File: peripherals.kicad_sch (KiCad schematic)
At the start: 20 parts, among them J2 Pad, Q1 MMBT3904, SW1 DSHP02TSGET, U2 BH1750FVI, U4 SHTC3

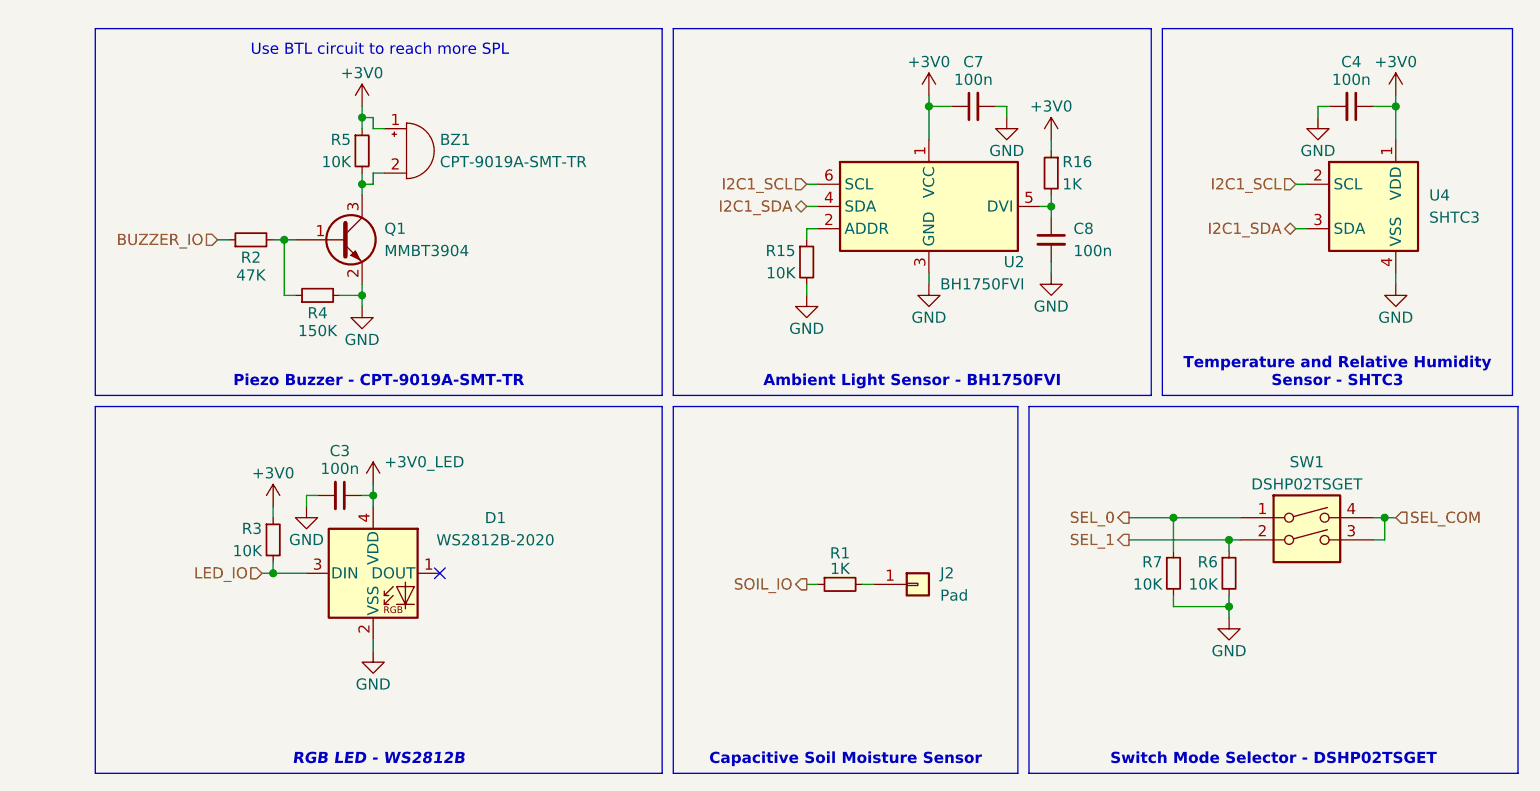
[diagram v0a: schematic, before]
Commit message: updated last changes
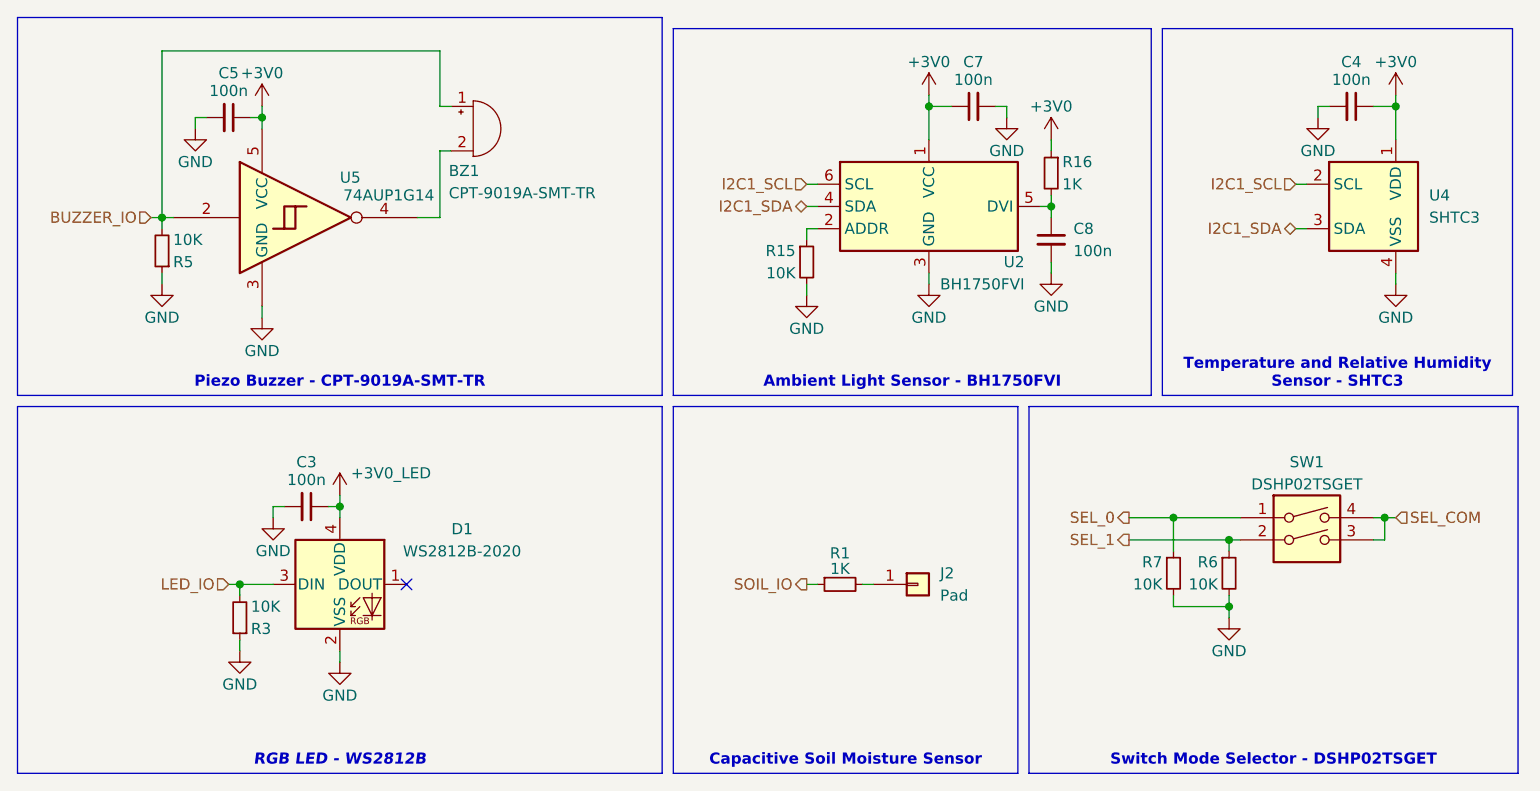
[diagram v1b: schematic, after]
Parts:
- removed Q1: MMBT3904, Package_TO_SOT_SMD:SOT-23, symbol Transistor_BJT:MMBT3904
- removed R2: 47K, Resistor_SMD:R_0603_1608Metric, symbol Device:R_Small
- removed R4: 150K, Resistor_SMD:R_0603_1608Metric, symbol Device:R_Small
- added C5: 100n, Capacitor_SMD:C_0603_1608Metric, symbol Device:C_Small
- added U5: 74AUP1G14, Package_TO_SOT_SMD:SOT-23-5, symbol 74xGxx:74AUP1G14
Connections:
- net +3V0: now also C5.1, U5.5 (VCC); no longer BZ1.1 (+), R3.1, R5.1
- net BUZZER_IO: now also BZ1.1 (+), R5.2, U5.2
- net GND: now also R3.1, R5.1, C5.2, U5.3 (GND)
- net at BZ1.2 (-): now also U5.4; no longer R5.2
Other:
- note removed: "Use BTL circuit to reach more SPL"
- moved on the sheet: BZ1, C3, D1, R3, R5
